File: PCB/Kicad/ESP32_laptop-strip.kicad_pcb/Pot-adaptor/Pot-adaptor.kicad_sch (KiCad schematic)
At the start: 2 parts, among them J1 Conn_01x03_Socket

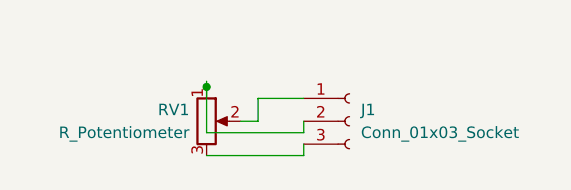
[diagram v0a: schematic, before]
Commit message: July2026
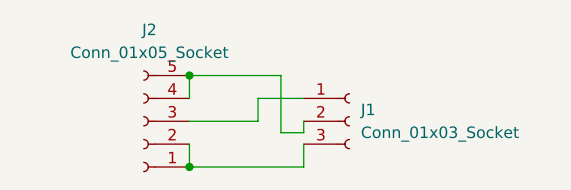
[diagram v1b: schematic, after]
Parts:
- removed RV1: R_Potentiometer, Connector_PinSocket_2.54mm:PinSocket_1x03_P2.54mm_Vertical, symbol Device:R_Potentiometer
- added J2: Conn_01x05_Socket, Connector_PinHeader_2.54mm:PinHeader_1x05_P2.54mm_Vertical, symbol Connector:Conn_01x05_Socket
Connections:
- net at J1.1 (Pin_1): now also J2.3 (Pin_3)
- net at J1.2 (Pin_2): now also J2.4 (Pin_4), J2.5 (Pin_5)
- net at J1.3 (Pin_3): now also J2.1 (Pin_1), J2.2 (Pin_2)
